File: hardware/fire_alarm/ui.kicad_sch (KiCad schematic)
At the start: 1 part

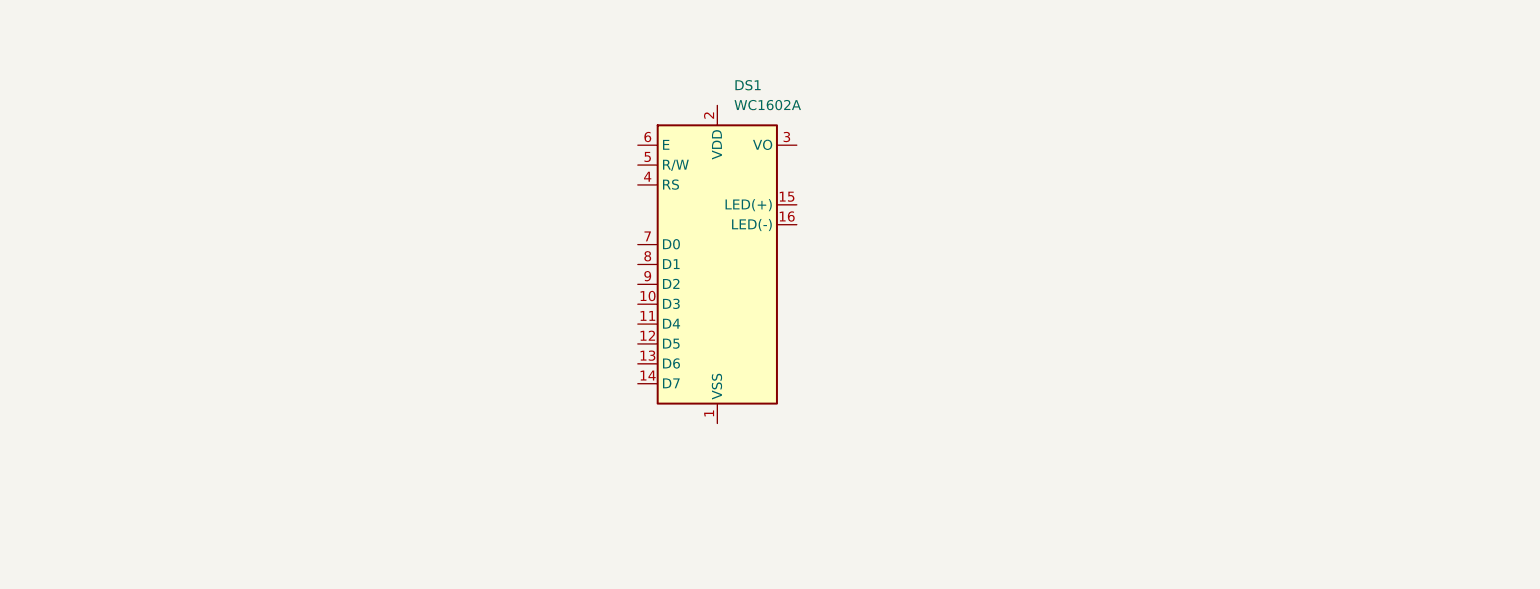
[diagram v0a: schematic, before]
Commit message: feat: complete schematic
Signed-off-by: Trung Hieu Nguyen <hieu.nguyenarc03@gmail.com>
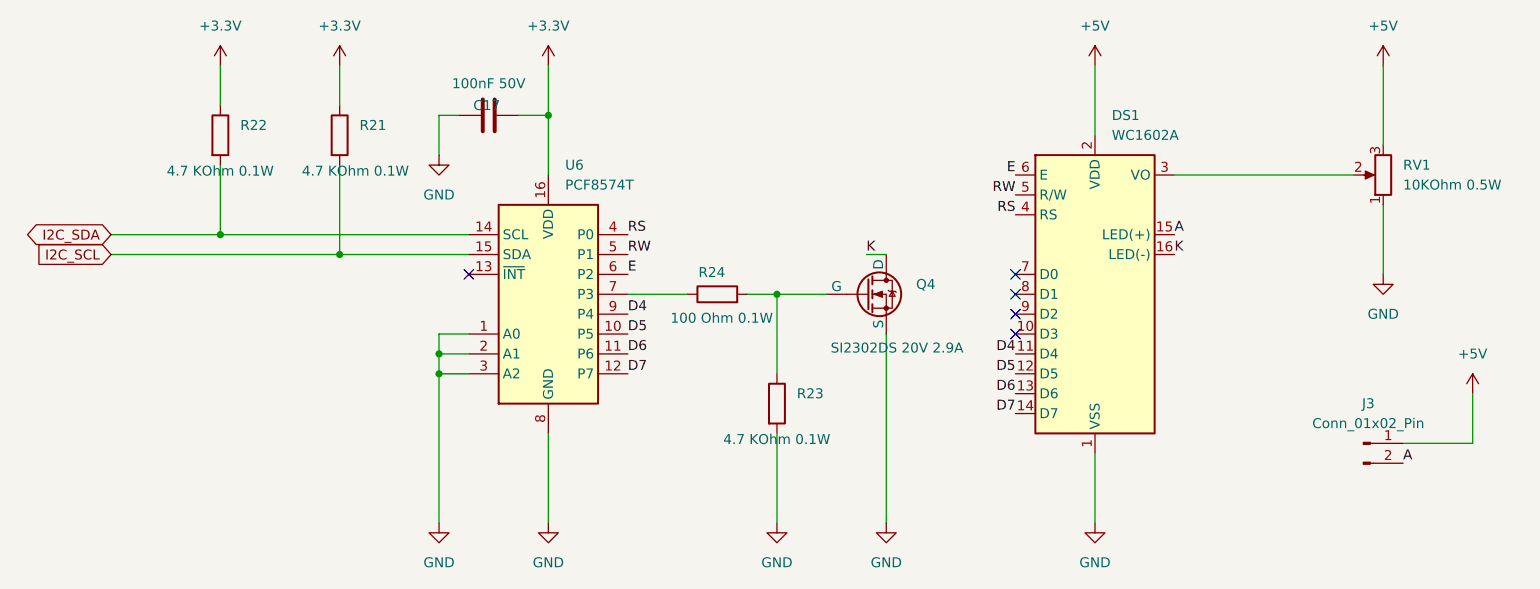
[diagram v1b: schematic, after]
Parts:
- added C17: 100nF 50V, Capacitor_SMD:C_0603_1608Metric_Pad1.08x0.95mm_HandSolder, symbol Device:C
- added J3: Conn_01x02_Pin, Connector_PinHeader_2.54mm:PinHeader_1x02_P2.54mm_Horizontal, symbol Connector:Conn_01x02_Pin
- added Q4: SI2302DS 20V 2.9A, Package_TO_SOT_SMD:SOT-23_Handsoldering, symbol Simulation_SPICE:NMOS
- added R21, R22, R23: 4.7 KOhm 0.1W, Resistor_SMD:R_0603_1608Metric_Pad0.98x0.95mm_HandSolder, symbol Device:R
- added R24: 100 Ohm 0.1W, Resistor_SMD:R_0603_1608Metric_Pad0.98x0.95mm_HandSolder, symbol Device:R
- added RV1: 10KOhm 0.5W, Potentiometer_THT:Potentiometer_Vishay_T73YP_Vertical, symbol Device:R_Potentiometer
- added U6: PCF8574T, Package_SO:SOIC-16W_7.5x10.3mm_P1.27mm, symbol Interface_Expansion:PCF8574T
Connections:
- net GND: now reaches DS1.1 (VSS)
- net GND: now also C17.1, Q4.3 (S), R23.2, RV1.1, U6.1 (A0), U6.2 (A1), U6.3 (A2), U6.8 (GND)
- net D4: now reaches DS1.11 (D4)
- net D4: now also U6.9 (P4)
- net D5: now reaches DS1.12 (D5)
- net D5: now also U6.10 (P5)
- net D6: now reaches DS1.13 (D6)
- net D6: now also U6.11 (P6)
- net D7: now reaches DS1.14 (D7)
- net D7: now also U6.12 (P7)
- net A: now reaches DS1.15 (LED(+))
- net A: now also J3.2 (Pin_2)
- net K: now reaches DS1.16 (LED(-))
- net K: now also Q4.1 (D)
- net +5V: now reaches DS1.2 (VDD)
- net +5V: now also J3.1 (Pin_1), RV1.3
- net at DS1.3 (VO): now also RV1.2
- net RS: now reaches DS1.4 (RS)
- net RS: now also U6.4 (P0)
- net RW: now reaches DS1.5 (R/W)
- net RW: now also U6.5 (P1)
- net E: now reaches DS1.6 (E)
- net E: now also U6.6 (P2)
- new net: Q4.2 (G), R23.1, R24.2
- new net: R24.1, U6.7 (P3)
- new net +3.3V: C17.2, R21.1, R22.1, U6.16 (VDD)
- new net I2C_SCL: R21.2, U6.15 (SDA)
- new net I2C_SDA: R22.2, U6.14 (SCL)
- no-connect marks 0 -> 5
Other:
- moved on the sheet: DS1
